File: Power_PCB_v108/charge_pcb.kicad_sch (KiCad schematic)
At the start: 42 parts, among them J1 Mow3, J10 Mot_Left, J11 DC/DC1, J12 DC/DC2, J2 Main_PCB1, J3 Mow2, J4 Battery, J5 Main_PCB2, J6 Power Switch, J7 Mow1, J8 Mot_Right, J9 Start, Q1 BC547C, Q2 IRF9540N, Q3 BC547C, Q4 IRF9540N, U1 INA226, U2 INA226, U3 INA226, U4 INA226, U5 INA226, U6 INA226

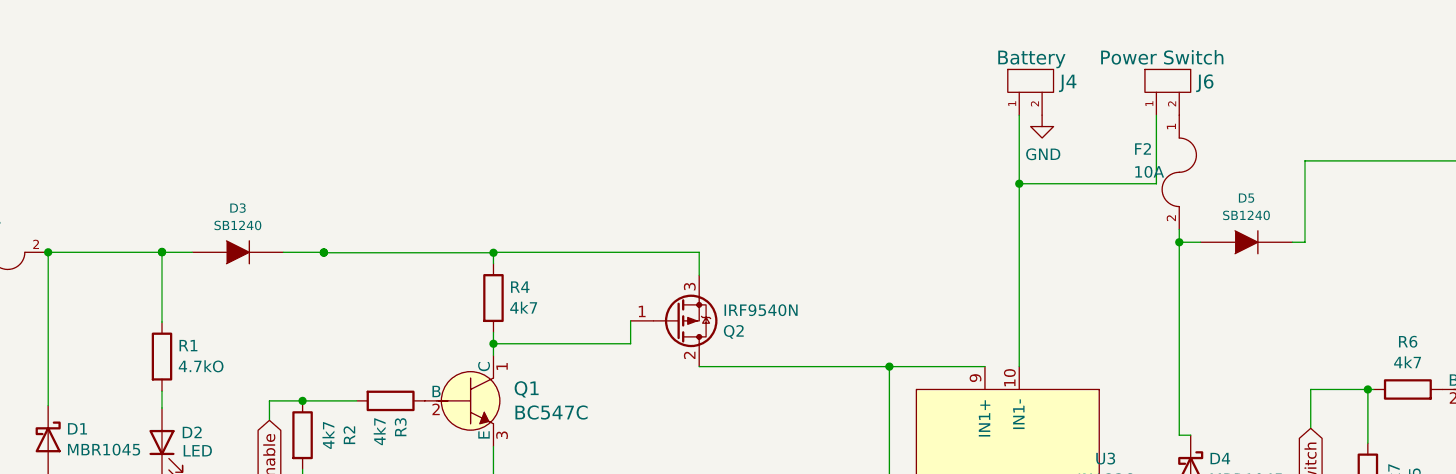
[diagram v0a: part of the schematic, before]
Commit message: Change Diode
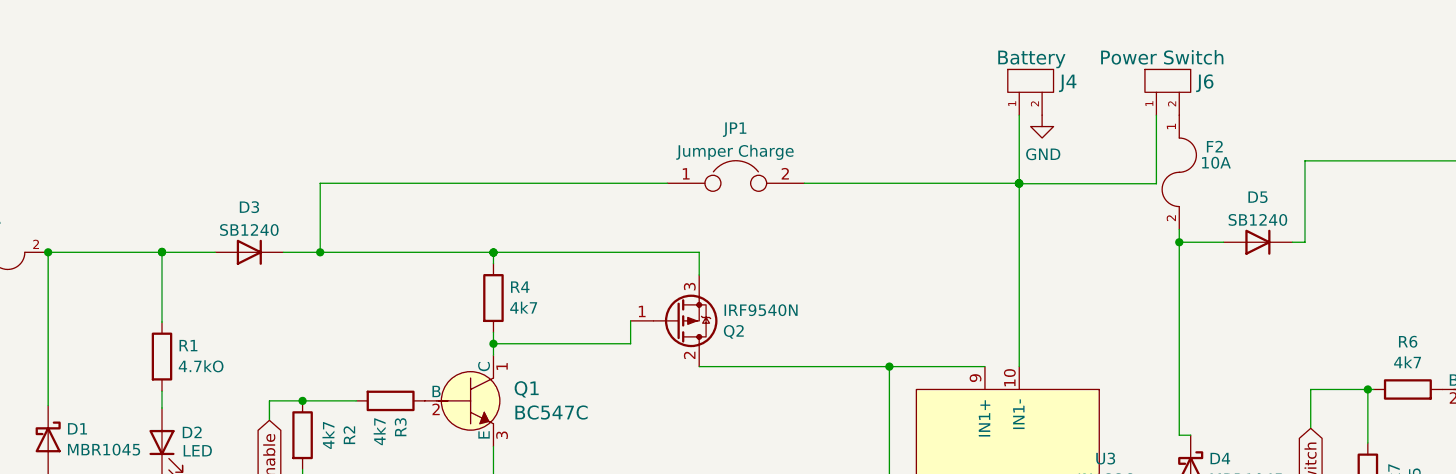
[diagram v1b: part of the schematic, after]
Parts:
- removed D3, D5: SB1240, Diode_THT:D_DO-41_SOD81_P10.16mm_Horizontal, symbol charge_pcb-rescue:DIODE-Lötpad_2,5mm-charge_pcb-rescue
- added D3, D5: SB1240, Diode_THT:D_DO-41_SOD81_P10.16mm_Horizontal, symbol Diode:1N5401
- added JP1: Jumper Charge, Connector_PinHeader_2.54mm:PinHeader_1x02_P2.54mm_Vertical, symbol Device:Jumper
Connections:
- net at D1.1 (K), F1.2, R1.1: now also D3.2 (A)
- net at Q2.3 (S), R4.1: now also D3.1 (K), JP1.1
- net at J4.1, J6.1, U3.10 (IN1-): now also JP1.2
- net at D4.1 (K), F2.2: now also D5.2 (A)
- net at Q4.3 (S), R7.1: now also D5.1 (K)
